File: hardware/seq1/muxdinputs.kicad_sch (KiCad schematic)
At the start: 20 parts, among them SW1 SW_Push, SW2 SW_Push, SW3 SW_Push, SW4 SW_Push, SW5 SW_Push, SW6 SW_Push, SW7 SW_Push, SW8 SW_Push, U2 74HC4051, U3 74HC4051

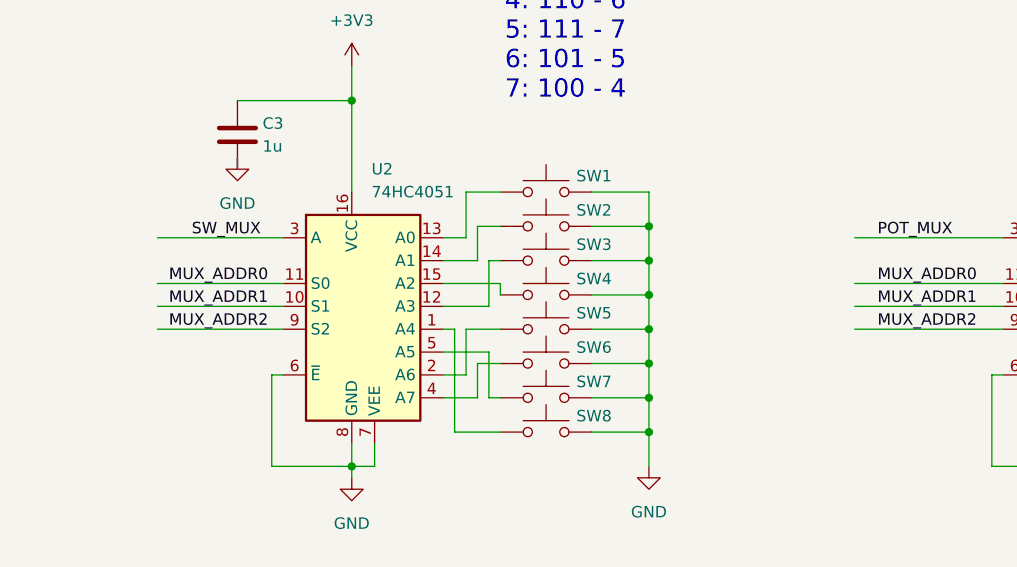
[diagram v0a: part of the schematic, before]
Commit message: schematic and layout for v1 board
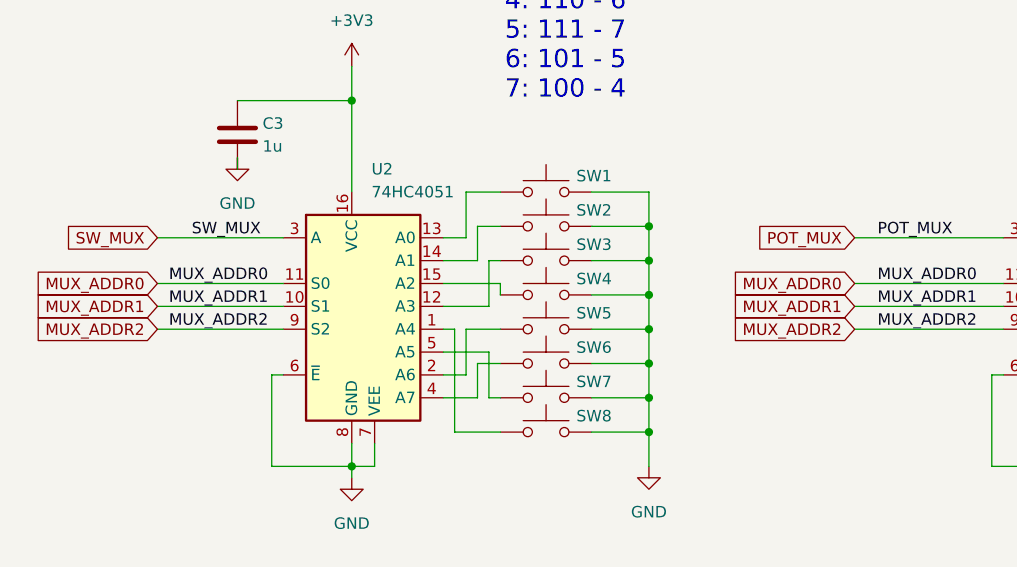
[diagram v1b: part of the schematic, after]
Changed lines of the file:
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@@
+		)
+	)
+	(global_label "MUX_ADDR1"
+		(shape input)
+		(at 36.83 95.25 180)
+		(fields_autoplaced yes)
+		(effects
+			(font
+				(size 1.27 1.27)
+			)
+			(justify right)
+		)
+		(property "Intersheetrefs" "${INTERSHEET_REFS}"
+			(at 22.7777 95.25 0)
+			(effects
+				(font
+					(size 1.27 1.27)
+				)
+				(justify right)
+				(hide yes)
+			)
+		)
+	)
+	(global_label "MUX_ADDR2"
+		(shape input)
+		(at 36.83 97.79 180)
+		(fields_autoplaced yes)
+		(effects
+			(font
+				(size 1.27 1.27)
+			)
+			(justify right)
+		)
+		(property "Intersheetrefs" "${INTERSHEET_REFS}"
+			(at 22.7777 97.79 0)
+			(effects
+				(font
+					(size 1.27 1.27)
+				)
+				(justify right)
+				(hide yes)
+			)
+		)
+	)
+	(global_label "MUX_ADDR2"
+		(shape input)
+		(at 114.3 97.79 180)
+		(fields_autoplaced yes)
+		(effects
+			(font
+				(size 1.27 1.27)
+			)
+			(justify right)
+		)
+		(property "Intersheetrefs" "${INTERSHEET_REFS}"
+			(at 100.2477 97.79 0)
+			(effects
+				(font
+					(size 1.27 1.27)
+				)
+				(justify right)
+				(hide yes)
+			)
+		)
+	)
+	(global_label "POT_MUX"
+		(shape input)
+		(at 114.3 87.63 180)
+		(fields_autoplaced yes)
+		(effects
+			(font
+				(size 1.27 1.27)
+			)
+			(justify right)
+		)
+		(property "Intersheetrefs" "${INTERSHEET_REFS}"
+			(at 102.7877 87.63 0)
+			(effects
+				(font
+					(size 1.27 1.27)
+				)
+				(justify right)
+				(hide yes)
+			)
+		)
+	)
+	(global_label "MUX_ADDR1"
+		(shape input)
+		(at 114.3 95.25 180)
+		(fields_autoplaced yes)
+		(effects
+			(font
+				(size 1.27 1.27)
+			)
+			(justify right)
+		)
+		(property "Intersheetrefs" "${INTERSHEET_REFS}"
+			(at 100.2477 95.25 0)
+			(effects
+				(font
+					(size 1.27 1.27)
+				)
+				(justify right)
+				(hide yes)
+			)
+		)
+	)
+	(global_label "SW_MUX"
+		(shape input)
+		(at 36.83 87.63 180)
+		(fields_autoplaced yes)
+		(effects
+			(font
+				(size 1.27 1.27)
+			)
+			(justify right)
+		)
+		(property "Intersheetrefs" "${INTERSHEET_REFS}"
+			(at 26.2249 87.63 0)
+			(effects
+				(font
+					(size 1.27 1.27)
+				)
+				(justify right)
+				(hide yes)
+			)
+		)
+	)
+	(global_label "MUX_ADDR0"
+		(shape input)
+		(at 36.83 92.71 180)
+		(fields_autoplaced yes)
+		(effects
+			(font
+				(size 1.27 1.27)
+			)
+			(justify right)
+		)
+		(property "Intersheetrefs" "${INTERSHEET_REFS}"
+			(at 22.7777 92.71 0)
+			(effects
+				(font
+					(size 1.27 1.27)
+				)
+				(justify right)
+				(hide yes)
+			)
+		)
+	)
+	(global_label "MUX_ADDR0"
+		(shape input)
+		(at 114.3 92.71 180)
+		(fields_autoplaced yes)
+		(effects
+			(font
+				(size 1.27 1.27)
+			)
+			(justify right)
+		)
+		(property "Intersheetrefs" "${INTERSHEET_REFS}"
+			(at 100.2477 92.71 0)
+			(effects
+				(font
+					(size 1.27 1.27)
+				)
+				(justify right)
+				(hide yes)
+			)
 		)
 	)
